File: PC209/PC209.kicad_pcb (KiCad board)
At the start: 2 copper layers, 90.5 x 36 mm, 79 parts, among them J1 PC209_BoardEdge_44pin, Q1 BC848W, Q10 BC848W, Q11 BC848W, Q12 BC848W, Q13 BC848W, Q14 BC848W, Q15 BC848W, Q16 BC848W, Q17 BC848W, Q2 BC848W, Q3 BC848W, Q4 BC848W, Q5 BC848W, Q6 BC848W, Q7 BC848W, Q8 BC848W, Q9 BC848W, U1 4010, U2 4010

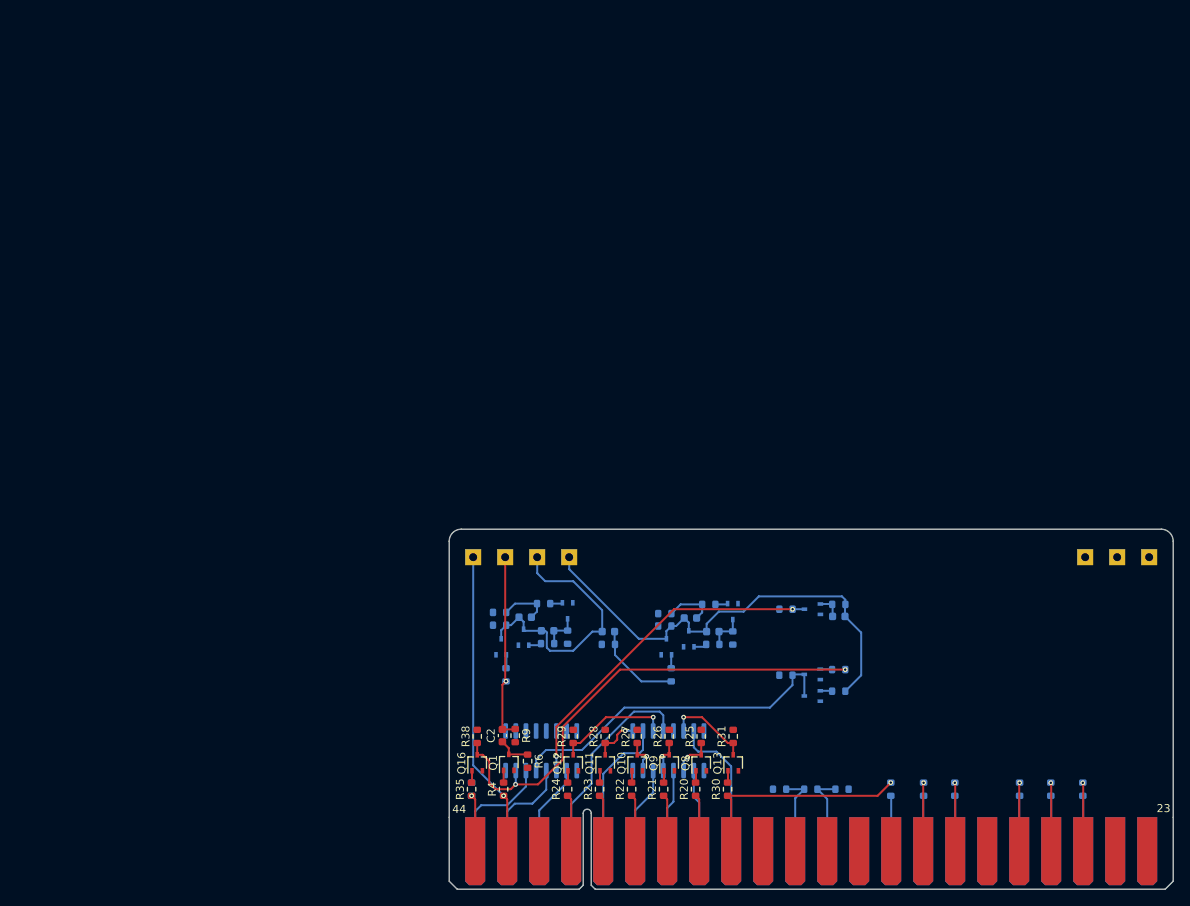
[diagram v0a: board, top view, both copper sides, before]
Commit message: PC209: Rev 1.0
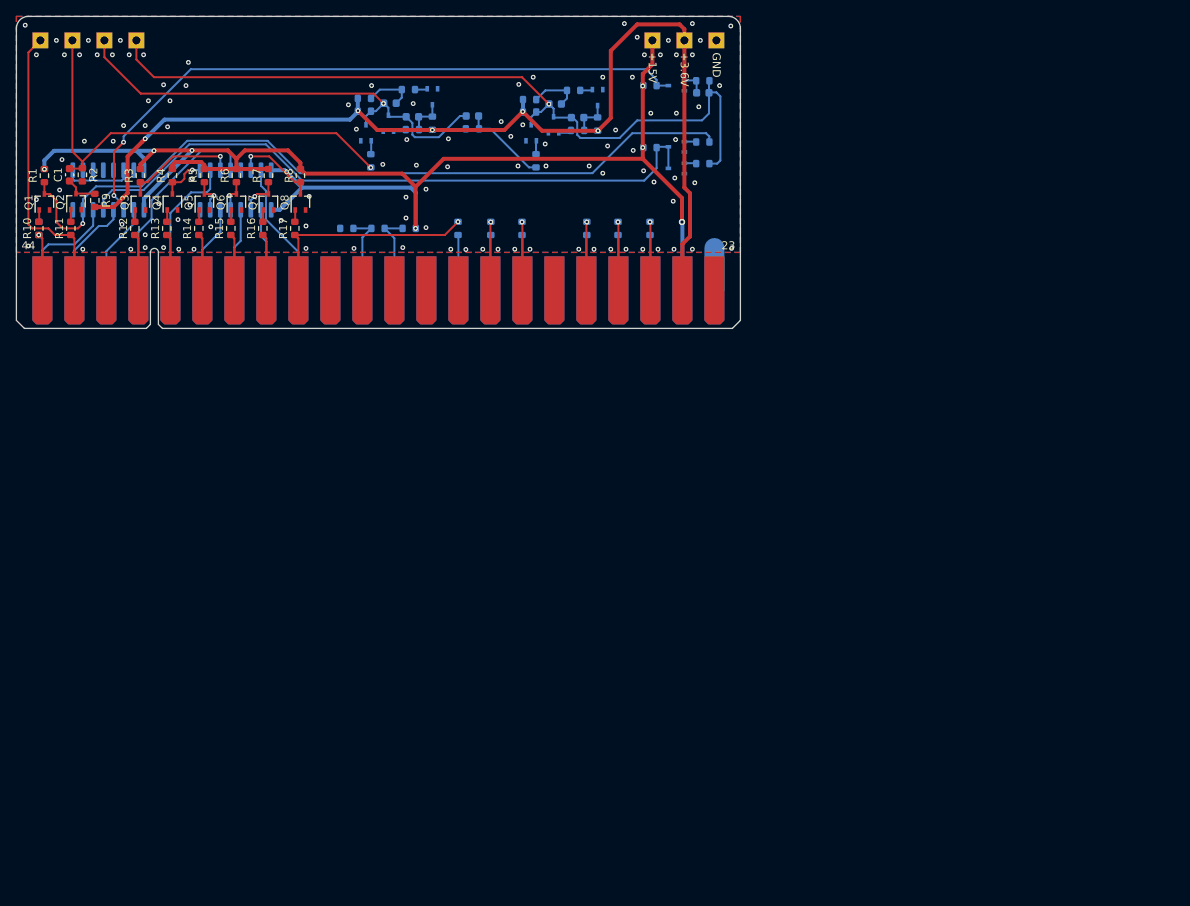
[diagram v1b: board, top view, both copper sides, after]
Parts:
- added REF**: OSHW-Logo_5.7x6mm_SilkScreen, Symbol:OSHW-Logo_5.7x6mm_SilkScreen, B.Cu at (89.9, 43.6)
- added REF**: KiCad-Logo2_5mm_SilkScreen, Symbol:KiCad-Logo2_5mm_SilkScreen, B.Cu at (79.9, 43.6)
- moved C1 88.5 mm to (56.5, 59.7)
- moved Q2 88.5 mm to (57.4, 63.0)
- moved R1 88.5 mm to (53.4, 59.8)
- moved R2 88.5 mm to (58.1, 59.7)
- moved R3 88.5 mm to (65.4, 59.8)
- moved R4 88.5 mm to (69.4, 59.8)
- moved R5 88.5 mm to (73.4, 59.8)
- moved R6 88.5 mm to (77.4, 59.8)
- moved R7 88.5 mm to (81.4, 59.8)
- moved R8 88.5 mm to (85.4, 59.8)
- moved J1 88.5 mm to (49.9, 69.9)
- moved Q1 88.5 mm to (53.4, 63.1)
- moved R15 88.5 mm to (76.7, 66.4)
- moved R16 88.5 mm to (80.7, 66.4)
- moved R17 88.5 mm to (84.7, 66.4)
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- renumbered C2 to C1, C7 to C2, C4 to C3, C6 to C4, C1 to C5, C3 to C6, C5 to C7, Q16 to Q1, Q6 to Q10, Q7 to Q11, Q5 to Q12, Q3 to Q13, Q2 to Q14, Q4 to Q15, Q17 to Q16, Q14 to Q17, Q1 to Q2, Q12 to Q3, Q11 to Q4, Q10 to Q5, Q9 to Q6, Q8 to Q7, Q13 to Q8, Q15 to Q9, R38 to R1, R35 to R10, R4 to R11, R24 to R12, R23 to R13, R22 to R14, R21 to R15, R20 to R16, R30 to R17, R33 to R18, R36 to R19, R9 to R2, R18 to R20, R14 to R21, R13 to R22, R17 to R23, R8 to R24, R12 to R25, R16 to R26, R19 to R27, R5 to R28, R15 to R29, R29 to R3, R10 to R30, R39 to R31, R37 to R32, R7 to R33, R11 to R34, R32 to R35, R40 to R36, R41 to R37, R42 to R38, R43 to R39, R28 to R4, R44 to R40, R45 to R41, R1 to R42, R2 to R43, R3 to R44, R34 to R45, R27 to R5, R26 to R6, R25 to R7, R31 to R8, R6 to R9, TP7 to TP1, TP6 to TP2, TP5 to TP3, TP2 to TP5, TP3 to TP6, TP1 to TP7
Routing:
- net +15V: track 0.00 -> 179.1 mm, vias 0 -> 7
- net +3.6V: track 0.00 -> 131.5 mm, vias 0 -> 5
- net /Pulse Generator/Output: track 58.3 -> 100.0 mm, vias 0 -> 1
- net Net-(Q15-Pad3): track 42.6 -> 83.0 mm
- net Net-(Q14-Pad3): track 42.7 -> 82.6 mm
- net Net-(Q16-Pad3): track 61.2 -> 98.9 mm, vias 2 -> 1
- net Net-(C2-Pad2): track 23.4 -> 57.4 mm
- net Net-(C1-Pad1): track 33.5 -> 57.9 mm, vias 0 -> 1
- net GND: track 0.00 -> 16.3 mm, vias 0 -> 107
- net Buffer Storage: track 38.5 -> 36.6 mm, vias 1 -> 0
- net Zero Check Print: track 18.3 -> 17.0 mm
- net Print CMD B: track 13.4 -> 12.7 mm
- net Net-(C1-Pad2): track 11.3 -> 10.7 mm
- added copper zone on B.Cu, net GND
- added copper zone on F.Cu, net GND
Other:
- board size 90.5 x 36 mm -> 90.5 x 30 mm
- board text added: "+15V"
- board text added: "+3.6V"
- board text added: "Delay"
- board text added: "GND"
- board text added: "Inv"
- board text added: "Keithley 615 PC209 Replacement V1.0 Peter Farley, 2023"
- board text added: "Pulse"
- board text added: "Store"
